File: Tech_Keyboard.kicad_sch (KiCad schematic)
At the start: 42 parts, among them SW1 RotaryEncoder_Switch_MP, U2 Arduino_Pro_Micro

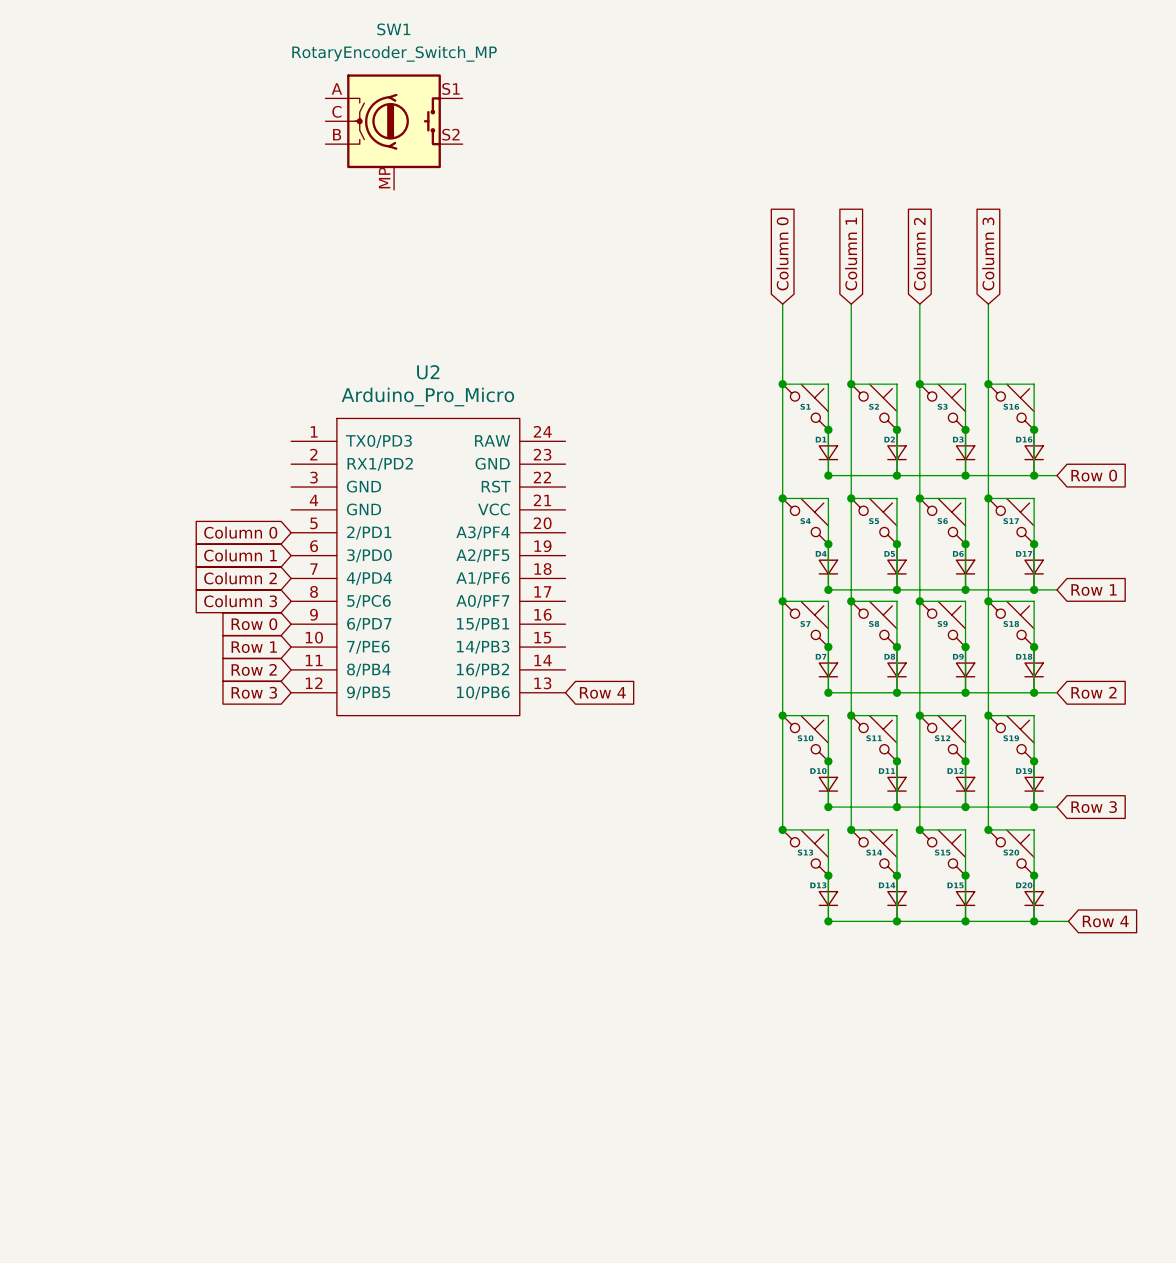
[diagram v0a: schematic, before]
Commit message: Update Tech_Keyboard.kicad_sch
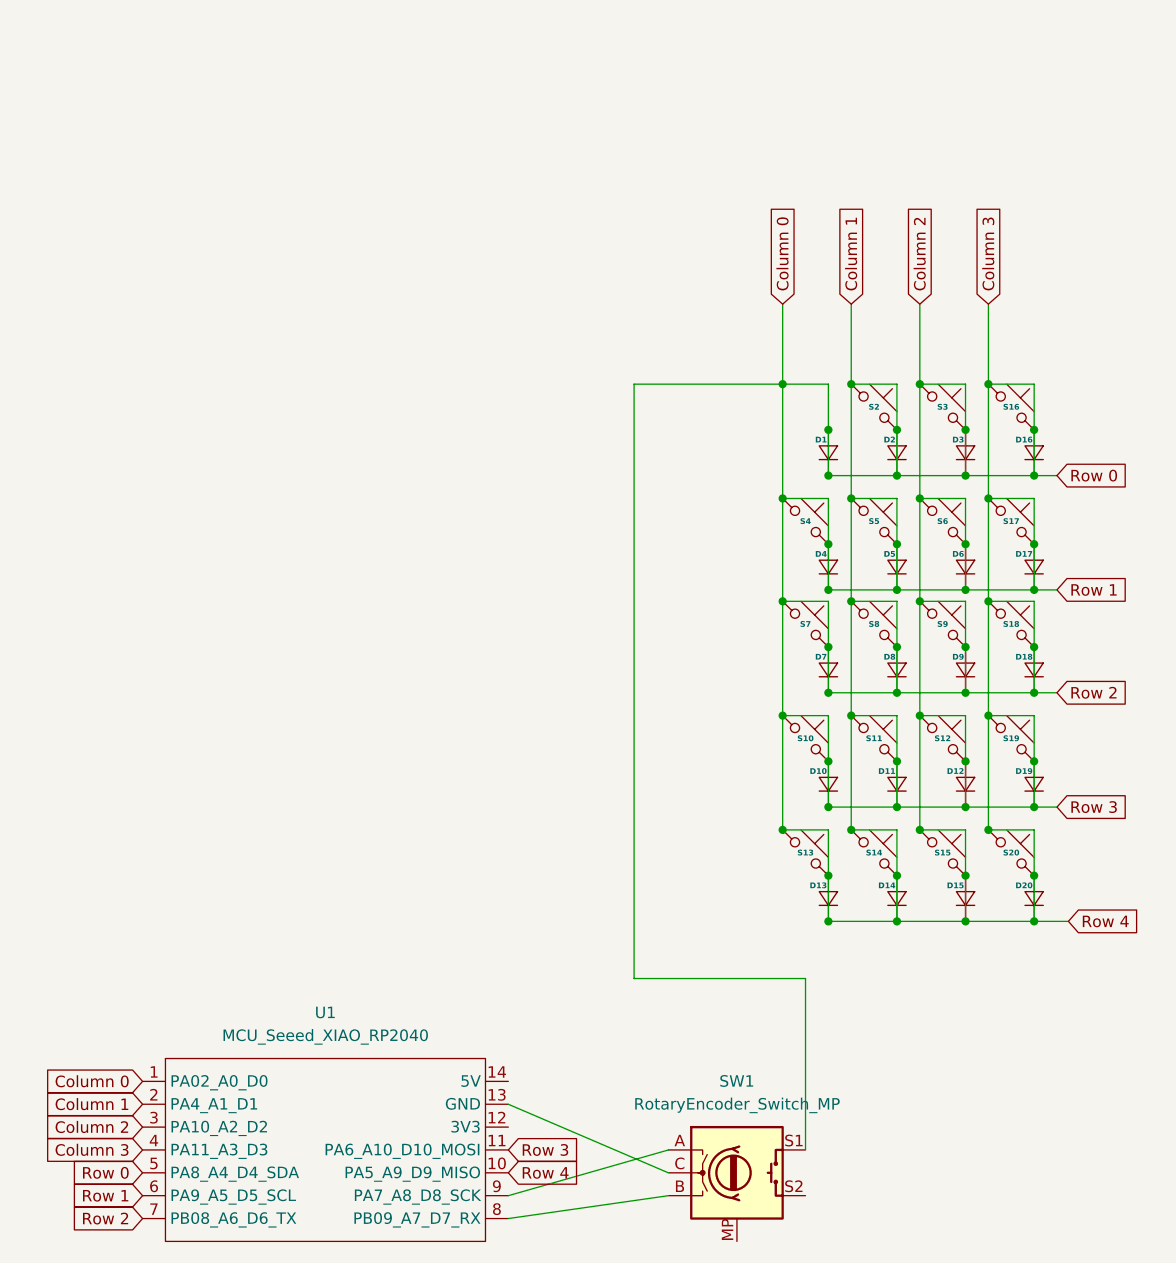
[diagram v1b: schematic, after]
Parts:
- removed S1: ~, symbol ScottoKeebs:Placeholder_Keyswitch
- removed U2: Arduino_Pro_Micro, ScottoKeebs_MCU:Arduino_Pro_Micro, symbol ScottoKeebs:MCU_Arduino_Pro_Micro
- added U1: MCU_Seeed_XIAO_RP2040, symbol ScottoKeebs:MCU_Seeed_XIAO_RP2040
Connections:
- net Column 0: now also SW1.S1, U1.1 (PA02_A0_D0), U1.10 (PA5_A9_D9_MISO), U1.11 (PA6_A10_D10_MOSI), U1.2 (PA4_A1_D1), U1.3 (PA10_A2_D2), U1.4 (PA11_A3_D3), U1.5 (PA8_A4_D4_SDA), U1.6 (PA9_A5_D5_SCL), U1.7 (PB08_A6_D6_TX)
- net at SW1.A: now also U1.9 (PA7_A8_D8_SCK)
- net at SW1.B: now also U1.8 (PB09_A7_D7_RX)
- net at SW1.C: now also U1.13 (GND)
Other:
- moved on the sheet: SW1
